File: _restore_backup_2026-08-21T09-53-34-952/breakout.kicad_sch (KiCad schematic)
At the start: 1 part, among them J1 Conn_02x05_Odd_Even

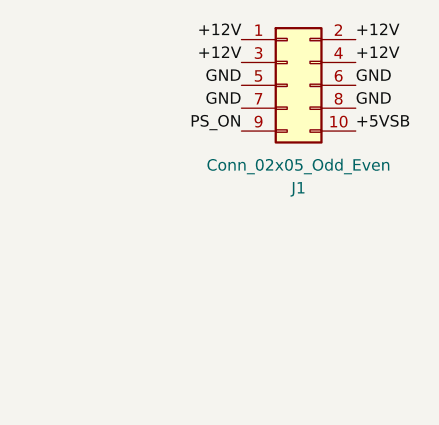
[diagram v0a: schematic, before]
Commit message: add readme
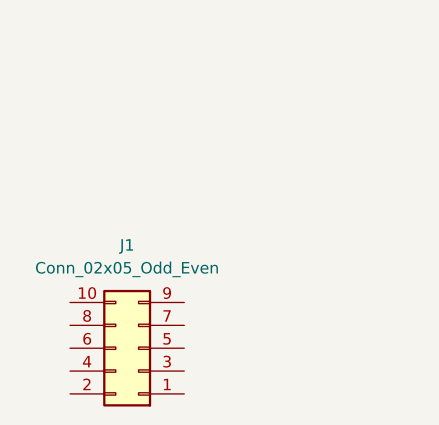
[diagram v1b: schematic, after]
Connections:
- removed net +12V: J1.1 (Pin_1), J1.2 (Pin_2), J1.3 (Pin_3), J1.4 (Pin_4)
- net +5VSB: no longer names the net of J1.10 (Pin_10)
- removed net GND: J1.5 (Pin_5), J1.6 (Pin_6), J1.7 (Pin_7), J1.8 (Pin_8)
- net PS_ON: no longer names the net of J1.9 (Pin_9)
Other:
- moved on the sheet: J1
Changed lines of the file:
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@@
 		(company "personal")
-	)
-	(label "+12V"
-		(at 60.96 91.44 180)
-		(effects
-			(font
-				(size 1.27 1.27)
-			)
-			(justify right bottom)
-		)
-	)
-	(label "GND"
-		(at 60.96 93.98 180)
-		(effects
-			(font
-				(size 1.27 1.27)
-			)
-			(justify right bottom)
-		)
-	)
-	(label "GND"
-		(at 73.66 93.98 0)
-		(effects
-			(font
-				(size 1.27 1.27)
-			)
-			(justify left bottom)
-		)
-	)
-	(label "+12V"
-		(at 73.66 91.44 0)
-		(effects
-			(font
-				(size 1.27 1.27)
-			)
-			(justify left bottom)
-		)
-	)
-	(label "GND"
-		(at 73.66 96.52 0)
-		(effects
-			(font
-				(size 1.27 1.27)
-			)
-			(justify left bottom)
-		)
-	)
-	(label "PS_ON"
-		(at 60.96 99.06 180)
-		(effects
-			(font
-				(size 1.27 1.27)
-			)
-			(justify right bottom)
-		)
-	)
-	(label "+12V"
-		(at 73.66 88.9 0)
-		(effects
-			(font
-				(size 1.27 1.27)
-			)
-			(justify left bottom)
-		)
-	)
-	(label "GND"
-		(at 60.96 96.52 180)
-		(effects
-			(font
-				(size 1.27 1.27)
-			)
-			(justify right bottom)
-		)
-	)
-	(label "+5VSB"
-		(at 73.66 99.06 0)
-		(effects
-			(font
-				(size 1.27 1.27)
-			)
-			(justify left bottom)
-		)
-	)
-	(label "+12V"
-		(at 60.96 88.9 180)
-		(effects
-			(font
-				(size 1.27 1.27)
-			)
-			(justify right bottom)
-		)
 	)
 	(symbol
 		(lib_id "Connector_Generic:Conn_02x05_Odd_Even")
-		(at 66.04 93.98 0)
+		(at 49.53 123.19 180)
 		(unit 1)
 		(body_style 1)
@@
 		(in_pos_files yes)
 		(dnp no)
+		(fields_autoplaced yes)
 		(property "Reference" "J1"
-			(at 67.31 105.41 0)
+			(at 48.26 111.76 0)
 			(show_name no)
 			(do_not_autoplace no)
@@
 		)
 		(property "Value" "Conn_02x05_Odd_Even"
-			(at 67.31 102.87 0)
+			(at 48.26 114.3 0)
 			(show_name no)
 			(do_not_autoplace no)
@@
 		)
 		(property "Footprint" ""
-			(at 66.04 93.98 0)
+			(at 49.53 123.19 0)
 			(hide yes)
 			(show_name no)
@@
 		)
 		(property "Datasheet" ""
-			(at 66.04 93.98 0)
+			(at 49.53 123.19 0)
 			(hide yes)
 			(show_name no)
@@
 		)
 		(property "Description" "Generic connector, double row, 02x05, odd/even pin numbering scheme (row 1 odd numbers, row 2 even numbers), script generated (kicad-library-utils/schlib/autogen/connector/)"
-			(at 66.04 93.98 0)
+			(at 49.53 123.19 0)
 			(hide yes)
 			(show_name no)
